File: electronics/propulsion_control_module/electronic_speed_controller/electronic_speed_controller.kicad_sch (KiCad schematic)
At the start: 46 parts, among them J1 Power, Q1 SiR696DP, Q2 SiR696DP, Q3 SiR696DP, Q4 SiR696DP, Q5 SiR696DP, Q6 SiR696DP, U1 STM32G071KBUxN, U2 HT7550-1-SOT89, U3 HT7533-1-SOT89, U4 DRV8300, U5 TPS7A45xxKTT, U6 INA180B1

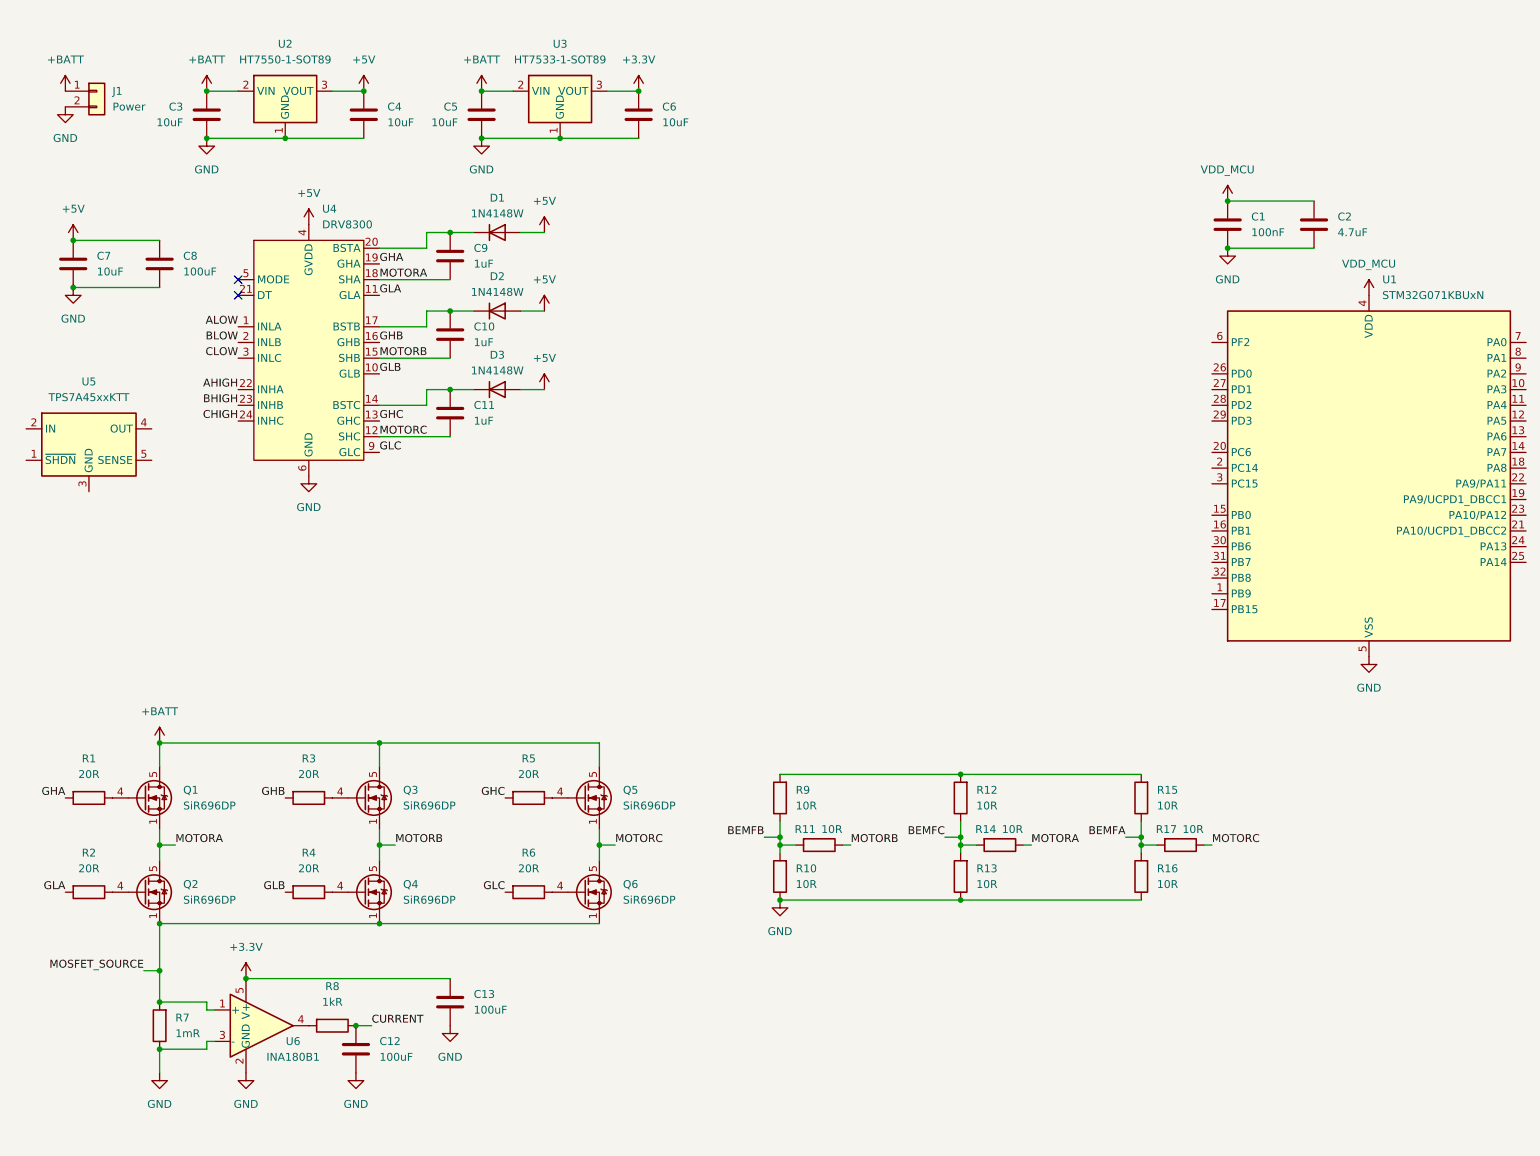
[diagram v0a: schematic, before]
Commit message: forgot to commit ESC schematic changes
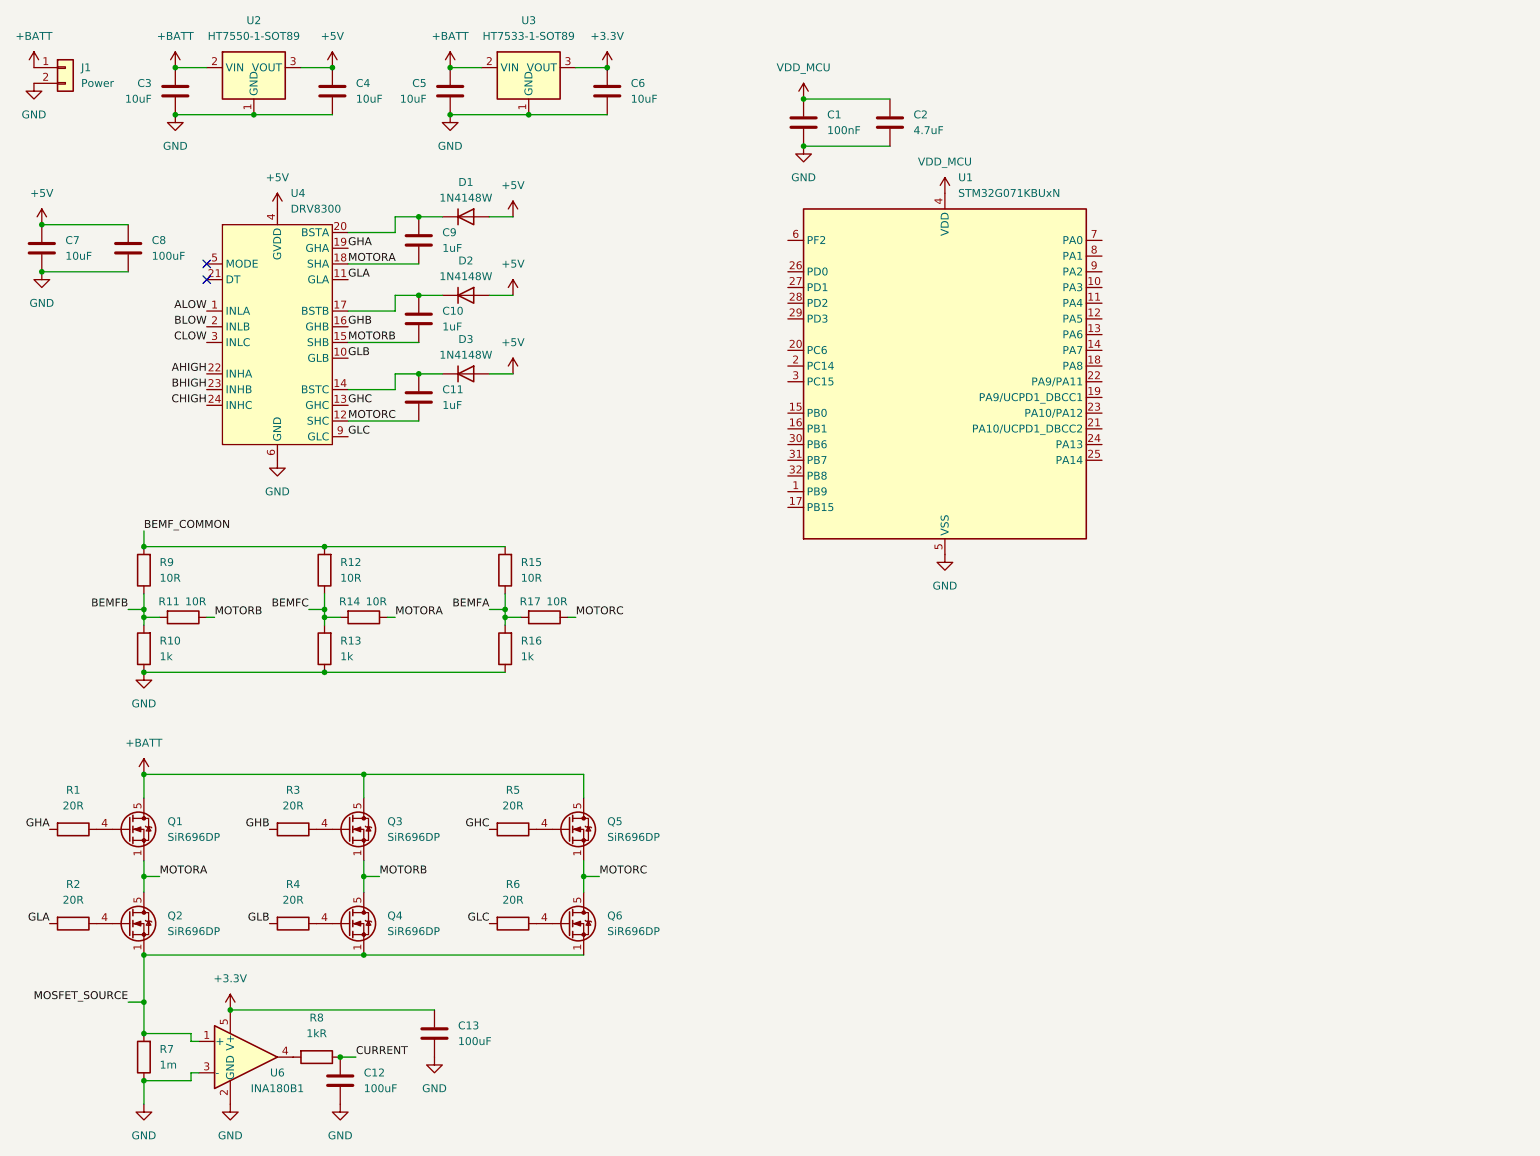
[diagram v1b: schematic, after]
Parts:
- removed U5: TPS7A45xxKTT, Package_TO_SOT_SMD:TO-263-5_TabPin3, symbol Regulator_Linear:TPS7A45xxKTT
- R10, R13, R16: value 10R -> 1k
- R7: value 1mR -> 1m
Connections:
- net BEMF_COMMON: now reaches R12.2, R15.2, R9.2
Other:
- moved on the sheet: C1, C10, C11, C12, C13, C2, C3, C4, C5, C6, C7, C8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
